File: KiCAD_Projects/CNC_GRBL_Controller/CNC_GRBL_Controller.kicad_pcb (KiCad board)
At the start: 2 copper layers, 85 x 50 mm, 17 parts, among them IC1 ATMEGA328-P, J1 DB25, P2 CONN_01X07, SW1 SW_PUSH_SMALL, U1 AE-UM232R, X1 CRYSTAL

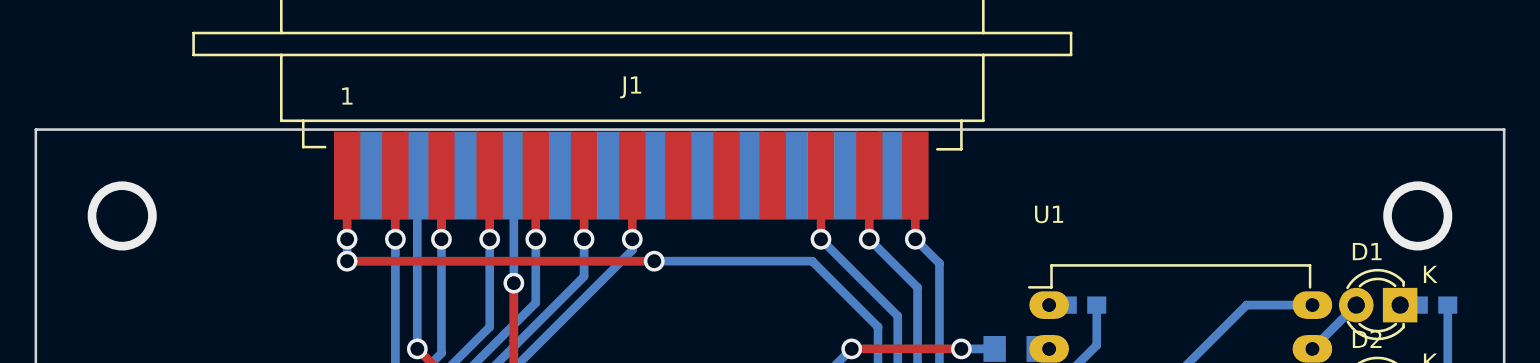
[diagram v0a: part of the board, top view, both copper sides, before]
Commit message: no message
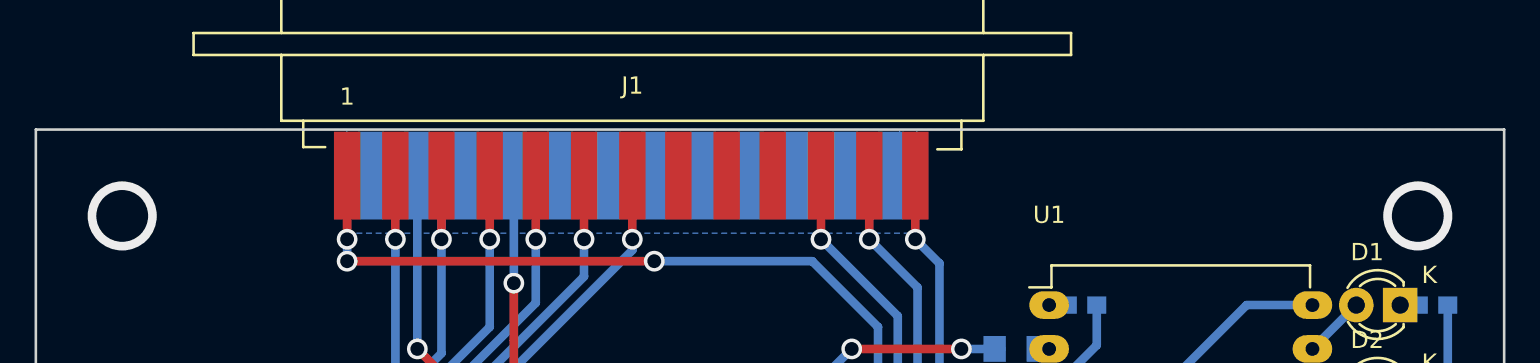
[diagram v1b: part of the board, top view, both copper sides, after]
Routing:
- added copper zone on B.Cu, net (none)
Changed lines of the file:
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@@
   (general
     (links 57)
-    (no_connects 0)
+    (no_connects 1)
     (area 14.924999 -0.075001 100.075001 50.075001)
     (thickness 1.6)
@@
   (segment (start 93.98 15.24) (end 95.035 15.24) (width 0.5) (layer B.Cu) (net 27))
   (segment (start 88.9 15.24) (end 91.44 15.24) (width 0.5) (layer B.Cu) (net 28))
-  (zone (net 2) (net_name GND) (layer B.Cu) (hatch edge 0.508)
+  (zone (net 0) (net_name "") (layer B.Cu) (hatch edge 0.508)
     (connect_pads (clearance 0.4))
     (min_thickness 0.2)
@@
     (polygon
       (pts
-        (xy 100 50) (xy 15 50) (xy 15 0) (xy 100 0) (xy 100 50)
+        (xy 100 0) (xy 100 50) (xy 15 50) (xy 15 0) (xy 33 0)
+        (xy 33 6) (xy 66 6) (xy 66 0)
       )
     )
+  )
+  (zone (net 2) (net_name GND) (layer B.Cu) (hatch edge 0.508)
+    (connect_pads yes (clearance 0.4))
+    (min_thickness 0.2)
+    (fill yes (arc_segments 16) (thermal_gap 0.508) (thermal_bridge_width 0.508))
+    (polygon
+      (pts
+        (xy 65 5) (xy 44 5) (xy 44 0) (xy 65 0) (xy 65 5)
+      )
+    )

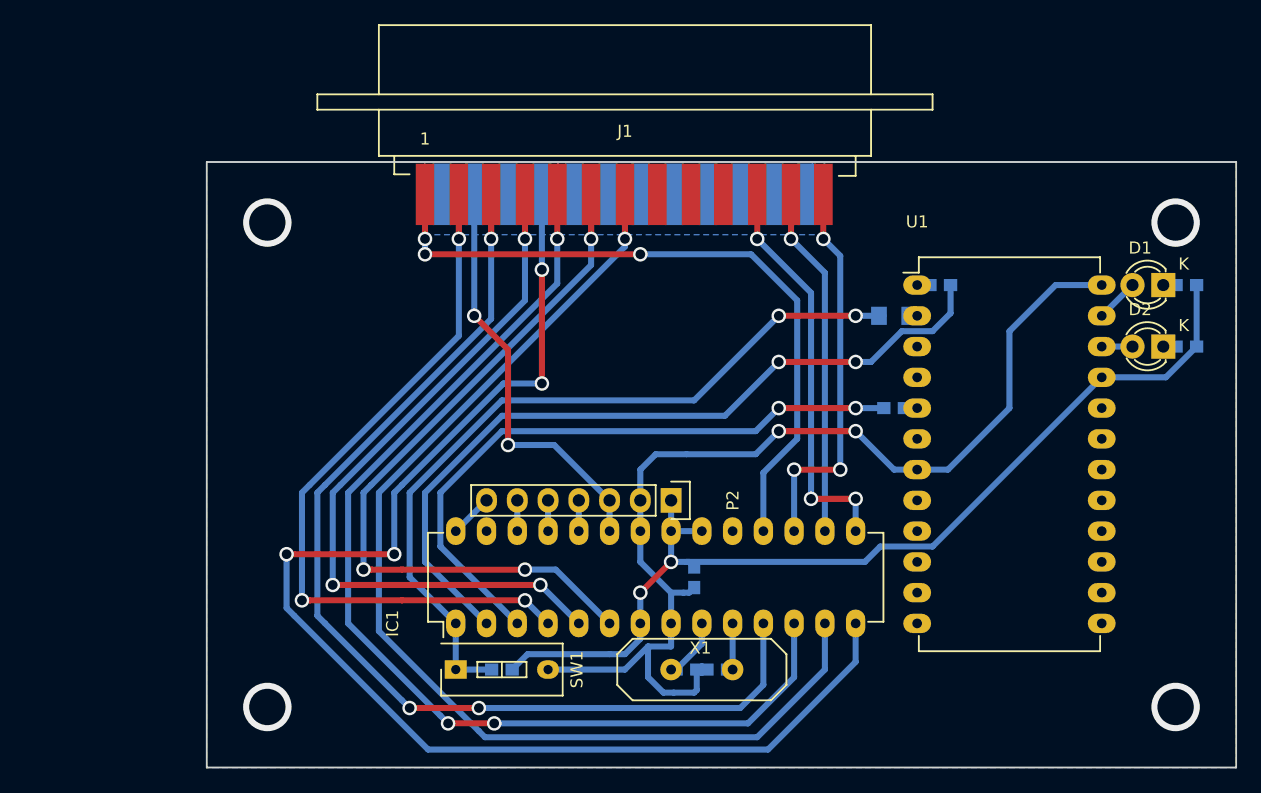
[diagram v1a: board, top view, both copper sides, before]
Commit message: no message
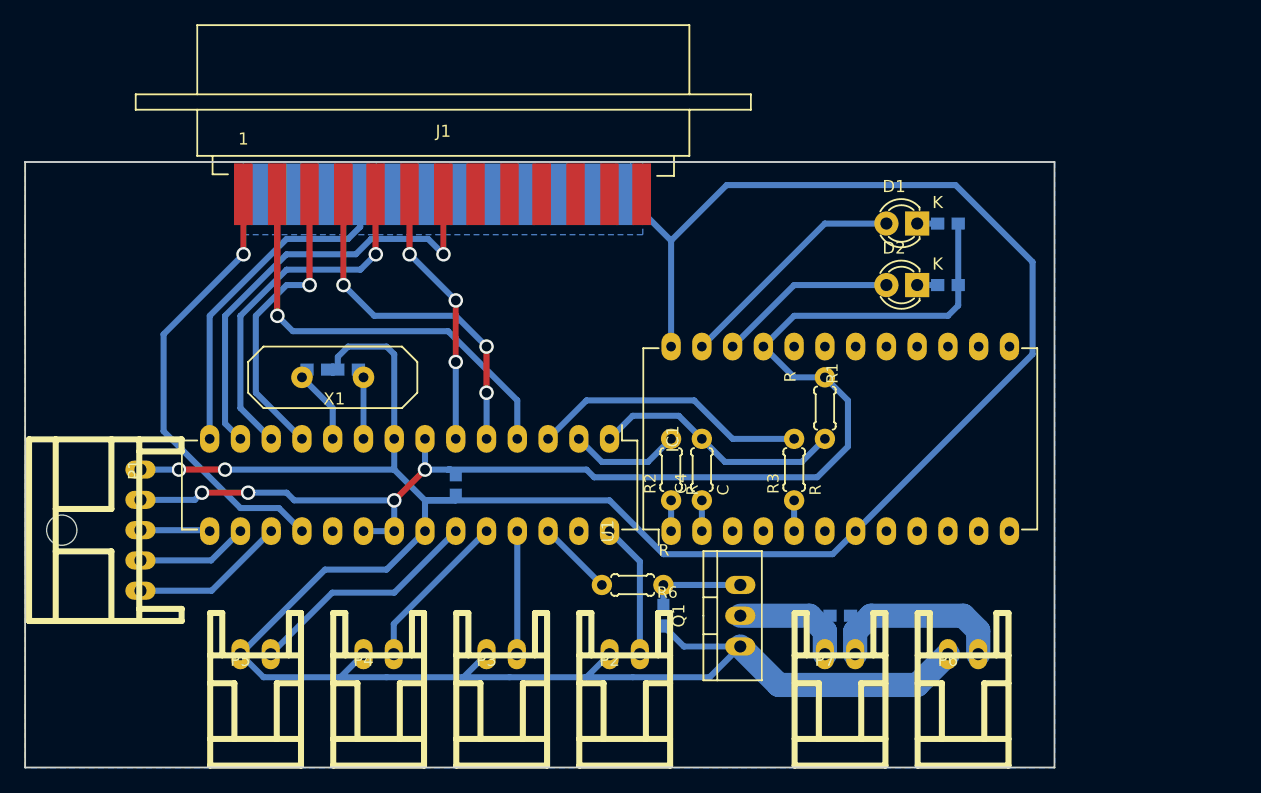
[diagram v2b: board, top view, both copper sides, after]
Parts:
- removed SW1: SW_PUSH_SMALL, Buttons_Switches_ThroughHole:SW_DIP_x1_Slide
- added C5: C, RP_KiCAD_Libs:C1608, B.Cu at (67.3, 37.5)
- added P1: CONN_01X05, RP_KiCAD_Connector:XA_5L, F.Cu at (9.53, 25.4)
- added P3: CONN_01X02, RP_KiCAD_Connector:XA_2L, F.Cu at (38.1, 40.6)
- added P4: CONN_01X02, RP_KiCAD_Connector:XA_2L, F.Cu at (27.9, 40.6)
- added P5: CONN_01X02, RP_KiCAD_Connector:XA_2L, F.Cu at (17.8, 40.6)
- added P6: CONN_01X02, RP_KiCAD_Connector:XA_2L, F.Cu at (76.2, 40.6)
- added P7: CONN_01X02, RP_KiCAD_Connector:XA_2L, F.Cu at (66.0, 40.6)
- added Q1: MOSFET_N, TO_SOT_Packages_THT:TO-220_Neutral123_Vertical, F.Cu at (59.1, 37.5)
- added R6: R, RP_KiCAD_Libs:0204_2f5, F.Cu at (50.2, 34.9)
- added R7: R, RP_KiCAD_Libs:C1608, B.Cu at (52.7, 37.5)
- C4: footprint RP_KiCAD_Libs:C2012 -> RP_KiCAD_Libs:0204_2f5; moved to F.Cu
- P2: value CONN_01X07 -> CONN_01X02; footprint Pin_Headers:Pin_Header_Straight_1x07 -> RP_KiCAD_Connector:XA_2L
- R1, R2, R3: footprint RP_KiCAD_Libs:C1608 -> RP_KiCAD_Libs:0204_2f5; moved to F.Cu
- moved C2 41.3 mm to (24.1, 17.1), turned to 180 degrees
- moved X1 38.9 mm to (25.4, 17.8), turned to 180 degrees
- moved C3 37.3 mm to (26.7, 17.1), turned to 0 degrees
- moved R1 34.3 mm to (66.0, 20.3), turned to 270 degrees
- moved U1 28.7 mm to (53.3, 30.5), turned to 90 degrees
- moved R2 26.9 mm to (53.3, 25.4), turned to 90 degrees
- moved C1 21.1 mm to (35.6, 26.7)
- moved D1 20.9 mm to (73.7, 5.08)
- moved D2 20.9 mm to (73.7, 10.2)
- moved R4 20.3 mm to (76.2, 5.08)
- moved R5 20.3 mm to (76.2, 10.2)
- moved C4 20.3 mm to (55.9, 25.4), turned to 90 degrees
- moved IC1 19.8 mm to (48.3, 22.9), turned to 270 degrees
- moved J1 15.0 mm to (34.5, 0.00)
- moved P2 13.7 mm to (48.3, 40.6), turned to 0 degrees
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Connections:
- J1 pad 11: /Limit_X -> (no net)
- J1 pad 12: /Limit_Y -> (no net)
- J1 pad 13: /Limit_Z -> (no net)
- J1 pad 15: /Reset/Abort -> (no net)
- P2 pad 1: +5V -> GND
- P2 pad 2: GND -> /Probe
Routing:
- net GND: track 89.5 -> 258.9 mm
- net /Stepper_~EN: track 108.0 -> 28.3 mm, vias 4 -> 0
- net /X_Dir: track 86.6 -> 24.7 mm, vias 3 -> 1
- net /Y_Dir: track 88.9 -> 29.5 mm, vias 3 -> 1
- net /Arduino_RX: track 64.8 -> 9.20 mm, vias 2 -> 0
- net /Z_Dir: track 91.1 -> 36.8 mm
- net /Arduino_RESET: track 64.3 -> 20.9 mm, vias 2 -> 0
- net /Z_Step: track 60.9 -> 21.8 mm
- net /Y_Step: track 60.5 -> 29.0 mm
- net /Arduino_TX: track 52.9 -> 23.0 mm, vias 2 -> 0
- net /Limit_X: track 33.3 -> 5.75 mm, vias 3 -> 0
- net +5V: track 83.6 -> 106.6 mm, vias 2 -> 4
- net /Spindle_EN: track 57.5 -> 37.1 mm, vias 3 -> 1
- net /Limit_Y: track 29.0 -> 9.26 mm, vias 1 -> 0
- net /Limit_Z: track 32.2 -> 12.8 mm, vias 3 -> 0
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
